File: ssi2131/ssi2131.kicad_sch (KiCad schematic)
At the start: 34 parts, among them J1 Saw Out, J2 Pulse Out, J3 Tri Out, J4 Hard Sync, J5 Soft Sync, J6 Expo Freq, J7 16-Pin uZeus Power Header, U1 SSI2131, U2 LM4040DBZ-2.5

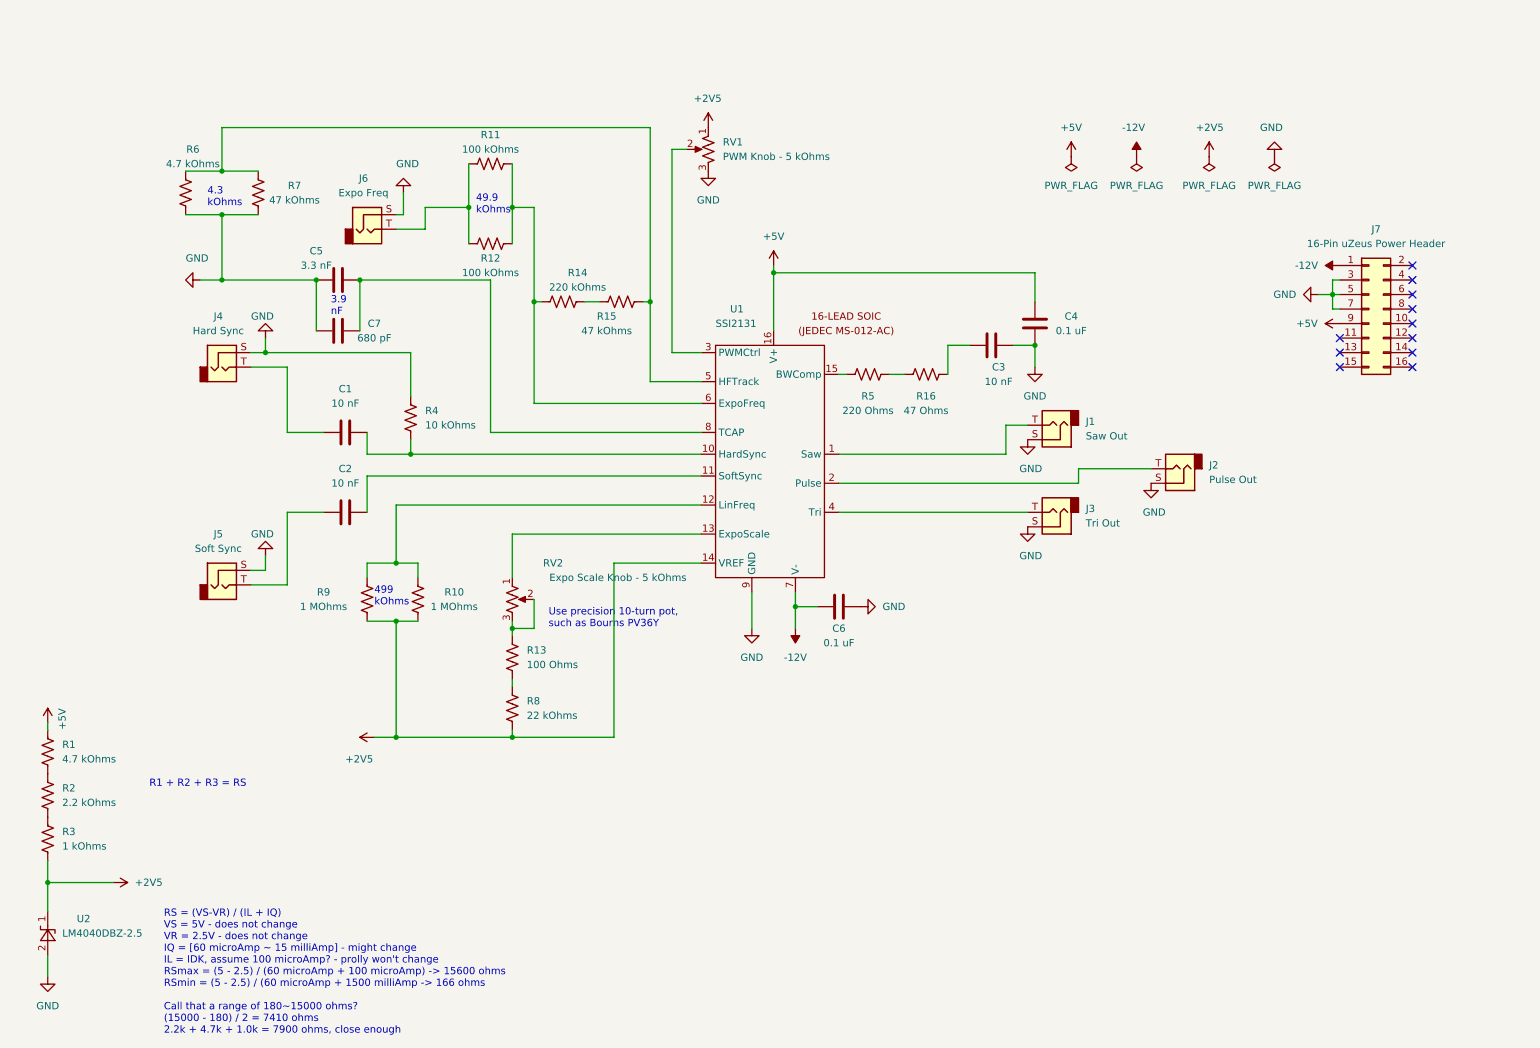
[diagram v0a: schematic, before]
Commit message: PCB attempt 1
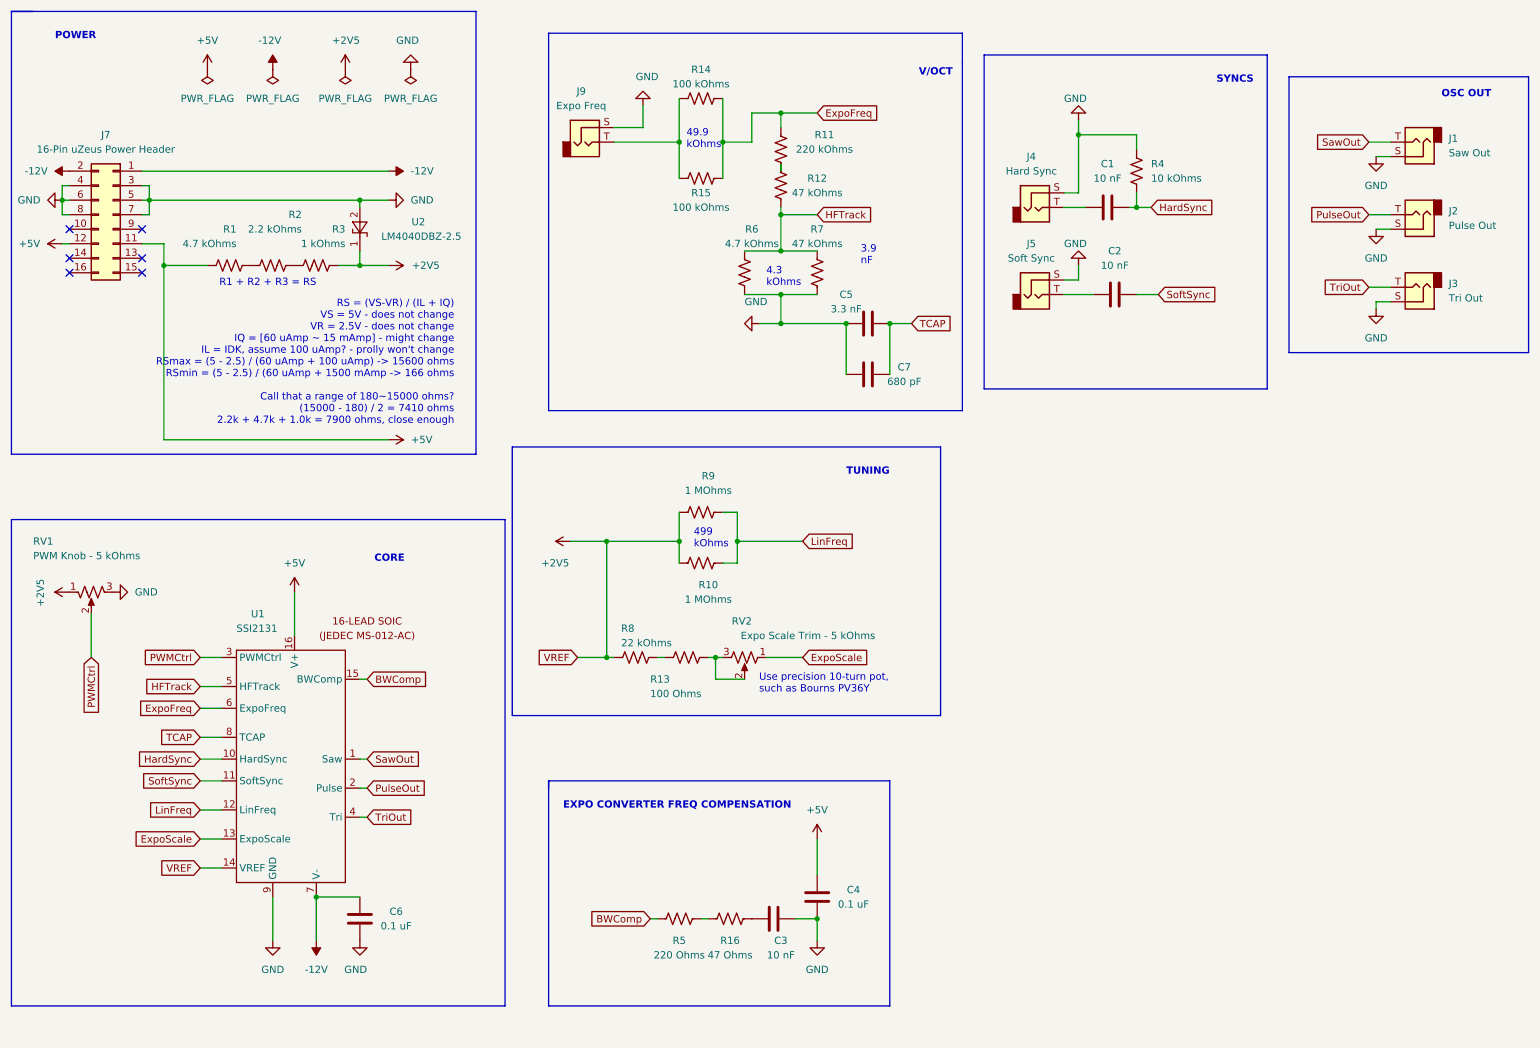
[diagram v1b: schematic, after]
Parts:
- removed J6: Expo Freq, Connector_Audio:Jack_3.5mm_QingPu_WQP-PJ398SM_Vertical_CircularHoles, symbol Connector:AudioJack2
- added J9: Expo Freq, Connector_Audio:Jack_3.5mm_QingPu_WQP-PJ398SM_Vertical_CircularHoles, symbol Connector:AudioJack2
- C1, C2, C3, C4, C5, C6, C7: footprint Capacitor_THT:C_Disc_D9.0mm_W2.5mm_P5.00mm -> Capacitor_THT:C_Disc_D6.0mm_W2.5mm_P5.00mm
- J7: footprint Connector_PinHeader_2.54mm:PinHeader_2x08_P2.54mm_Horizontal -> Connector_PinHeader_2.54mm:PinHeader_2x08_P2.54mm_Vertical
- R1, R10, R13, R16, R2, R3, R4, R5, R6, R7, R8, R9: footprint Resistor_THT:R_Axial_DIN0207_L6.3mm_D2.5mm_P10.16mm_Horizontal -> Resistor_THT:R_Axial_DIN0207_L6.3mm_D2.5mm_P2.54mm_Vertical
- R11: value 100 kOhms -> 220 kOhms; footprint Resistor_THT:R_Axial_DIN0207_L6.3mm_D2.5mm_P10.16mm_Horizontal -> Resistor_THT:R_Axial_DIN0207_L6.3mm_D2.5mm_P2.54mm_Vertical
- R12: value 100 kOhms -> 47 kOhms; footprint Resistor_THT:R_Axial_DIN0207_L6.3mm_D2.5mm_P10.16mm_Horizontal -> Resistor_THT:R_Axial_DIN0207_L6.3mm_D2.5mm_P2.54mm_Vertical
- R14: value 220 kOhms -> 100 kOhms; footprint Resistor_THT:R_Axial_DIN0207_L6.3mm_D2.5mm_P10.16mm_Horizontal -> Resistor_THT:R_Axial_DIN0207_L6.3mm_D2.5mm_P2.54mm_Vertical
- R15: value 47 kOhms -> 100 kOhms; footprint Resistor_THT:R_Axial_DIN0207_L6.3mm_D2.5mm_P10.16mm_Horizontal -> Resistor_THT:R_Axial_DIN0207_L6.3mm_D2.5mm_P2.54mm_Vertical
- RV2: value Expo Scale Knob - 5 kOhms -> Expo Scale Trim - 5 kOhms
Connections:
- net +5V: now also J7.11 (Pin_11), J7.12 (Pin_12); no longer J7.9 (Pin_9)
- net -12V: now also J7.2 (Pin_2)
- net GND: now also J7.4 (Pin_4), J7.6 (Pin_6), J7.8 (Pin_8), J9.S
- net HardSync: now reaches C1.2, R4.2, U1.10 (HardSync)
- net at R15.1: now also R14.1, J9.T; no longer R14.2
- net HFTrack: now reaches R6.1, R7.1, U1.5 (HFTrack)
- net HFTrack: now also R12.1; no longer R15.2
- net SawOut: now reaches J1.T, U1.1 (Saw)
- net at R11.1: now also R12.2; no longer R12.1
- net ExpoFreq: now reaches R11.2, U1.6 (ExpoFreq)
- net ExpoFreq: now also R14.2, R15.2; no longer R12.2, R14.1
- net TCAP: now reaches C5.1, C7.1, U1.8 (TCAP)
- net BWComp: now reaches R5.1, U1.15 (BWComp)
- net LinFreq: now reaches R10.2, R9.2, U1.12 (LinFreq)
- net SoftSync: now reaches C2.1, U1.11 (SoftSync)
- net ExpoScale: now reaches RV2.1, U1.13 (ExpoScale)
- net PulseOut: now reaches J2.T, U1.2 (Pulse)
- net PWMCtrl: now reaches RV1.2, U1.3 (PWMCtrl)
- net TriOut: now reaches J3.T, U1.4 (Tri)
- no-connect marks 11 -> 6
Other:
- note added: "CORE"
- note added: "EXPO CONVERTER FREQ COMPENSATION"
- note added: "OSC OUT"
- note added: "POWER"
- note added: "RS = (VS-VR) / (IL + IQ) VS = 5V - does not change VR = 2.5V - does not change IQ = [60 uAmp ~ 15 mAmp] - might change IL = IDK, assume 100 uAmp? - prolly won't change RSmax = (5 - 2.5) / (60 uAmp + 100 uAmp) -> 15600 ohms RSmin = (5 - 2.5) / (60 uAmp + 1500 mAmp -> 166 ohms Call that a range of 180~15000 ohms? (15000 - 180) / 2 = 7410 ohms 2.2k + 4.7k + 1.0k = 7900 ohms, close enough"
- note added: "SYNCS"
- note added: "TUNING"
- note added: "V/OCT"
- note removed: "RS = (VS-VR) / (IL + IQ) VS = 5V - does not change VR = 2.5V - does not change IQ = [60 microAmp ~ 15 milliAmp] - might change IL = IDK, assume 100 microAmp? - prolly won't change RSmax = (5 - 2.5) / (60 microAmp + 100 microAmp) -> 15600 ohms RSmin = (5 - 2.5) / (60 microAmp + 1500 milliAmp -> 166 ohms Call that a range of 180~15000 ohms? (15000 - 180) / 2 = 7410 ohms 2.2k + 4.7k + 1.0k = 7900 oh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"
- moved on the sheet: C1, C2, C5, C6, C7, J1, J2, J3, J4, J5, J7, R10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
